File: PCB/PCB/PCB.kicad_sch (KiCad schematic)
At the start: 53 parts, among them J1 AudioJack Right, J2 USB_B_Micro, J3 AudioJack Left, J4 6PIN DISPLAY CONNECTOR, J5 CONN BAT, Q1 BC817, Q2 BC817, Q3 BSS84, U1 ESP32-S3-WROOM-1, U2 CP2102N-Axx-xQFN28, U3 NCP1117-3.3_SOT223, U4 UDA1334ATS, U5 PAM8403D, U6 MCP73831-3-OT

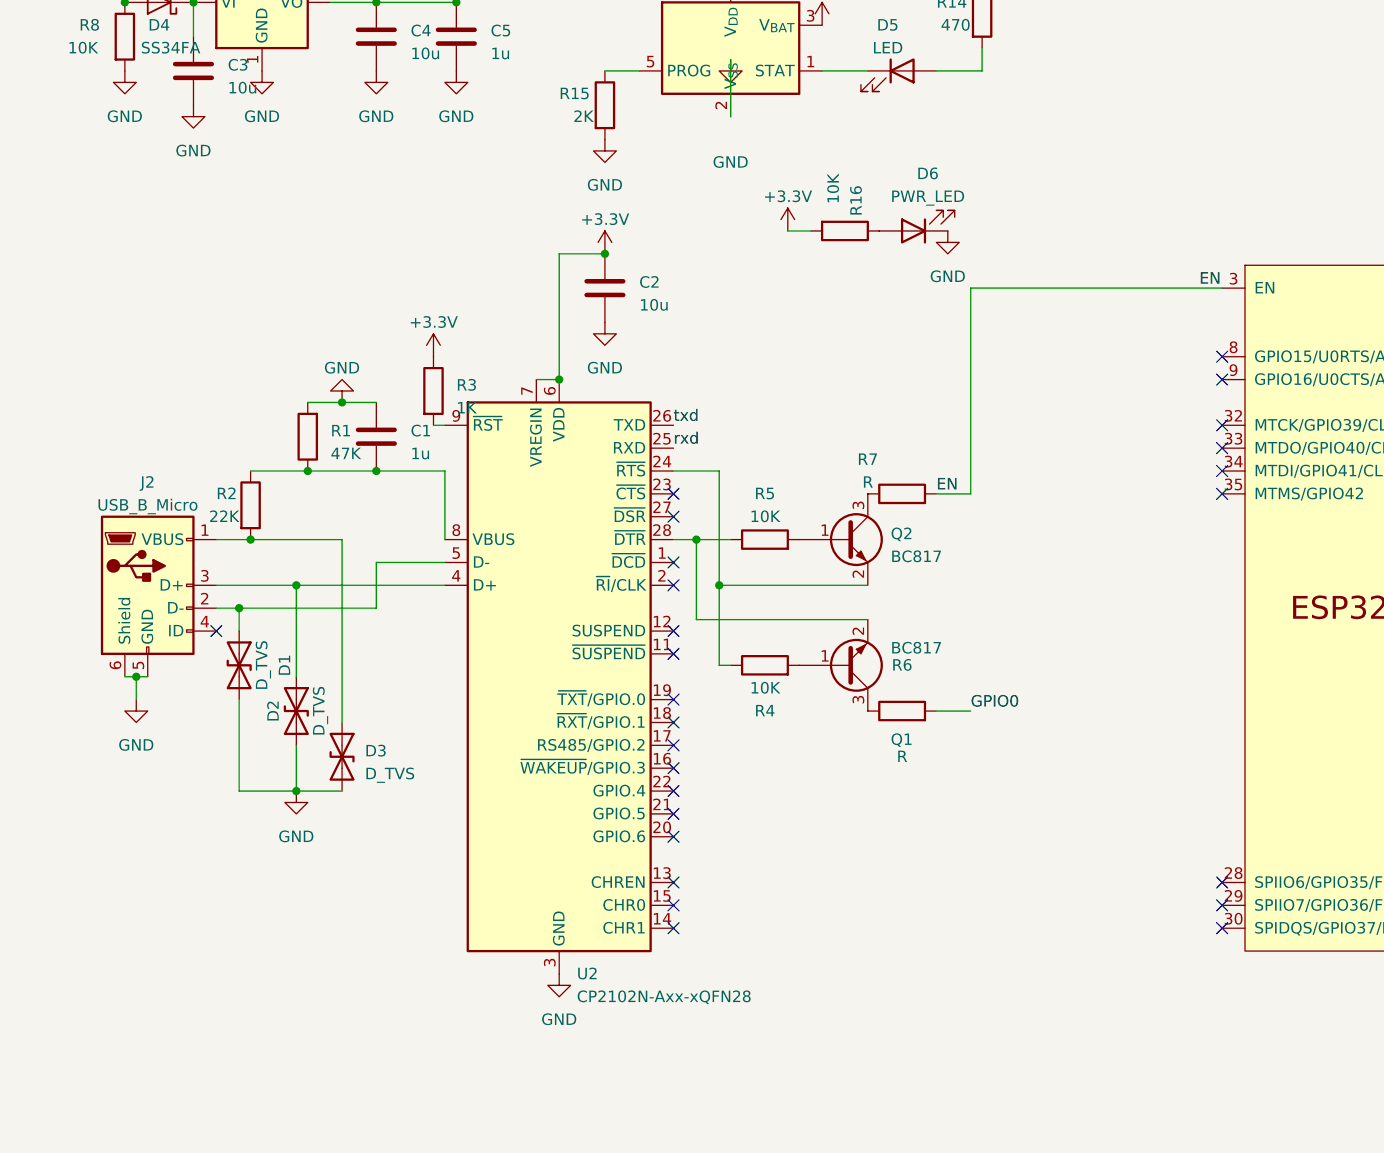
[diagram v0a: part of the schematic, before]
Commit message: PCB finished
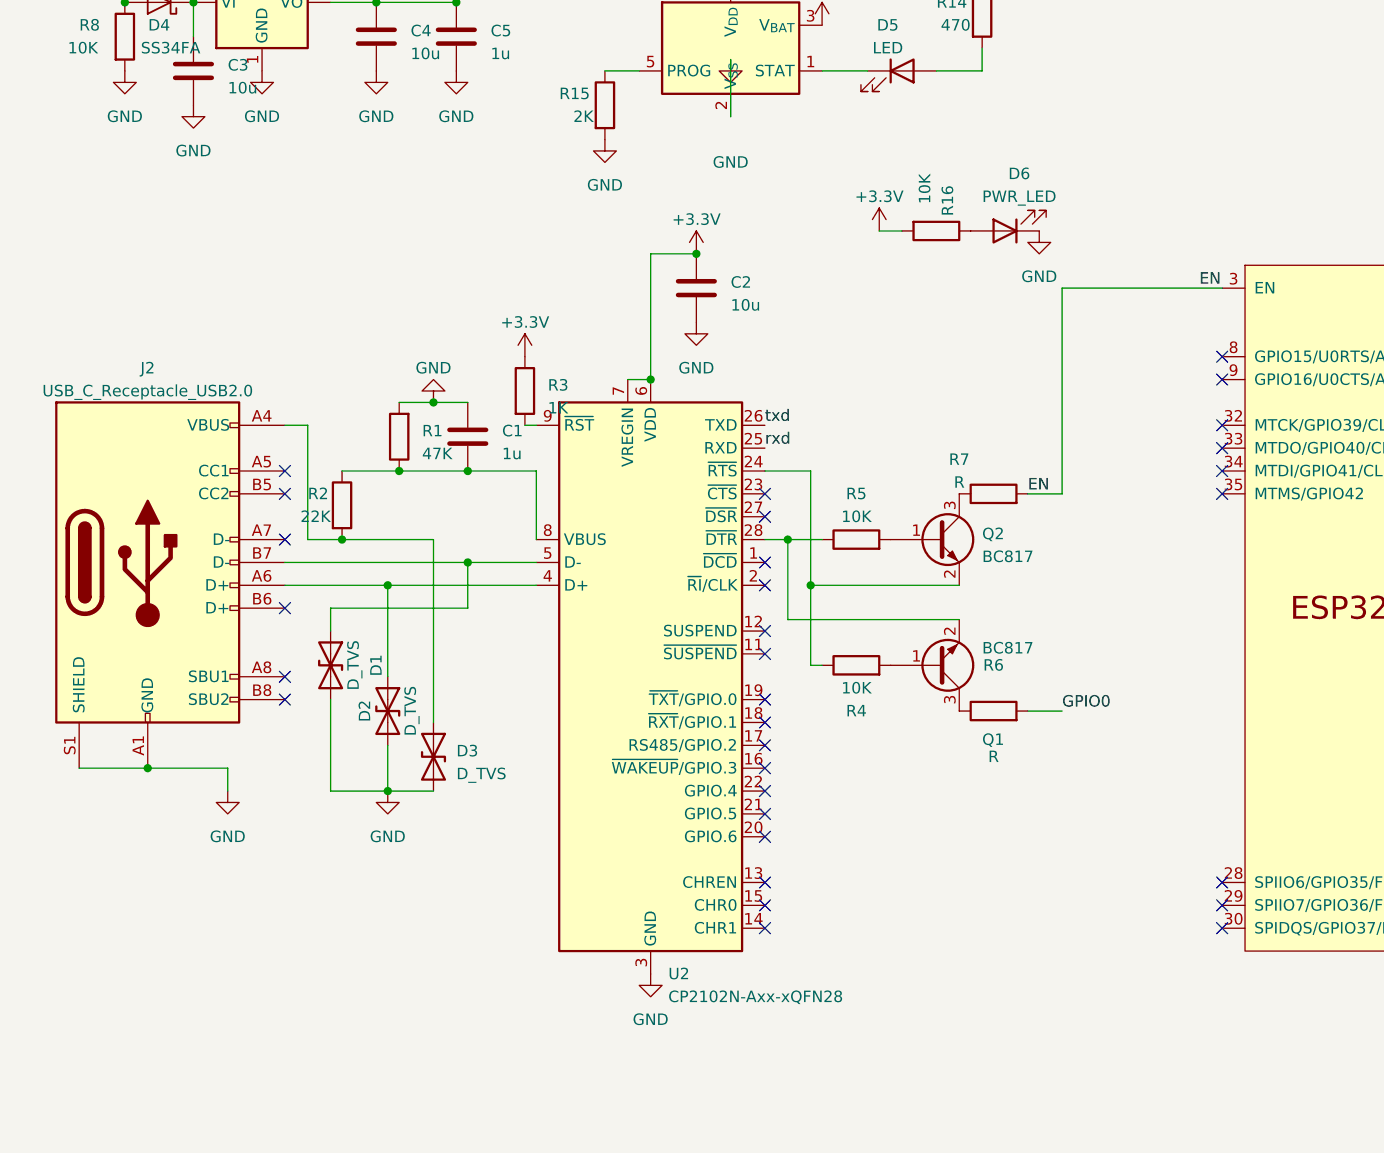
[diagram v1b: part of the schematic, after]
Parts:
- removed J2: USB_B_Micro, Connector_USB:USB_Micro-B_Molex-105017-0001, symbol Connector:USB_B_Micro
- added J2: USB_C_Receptacle_USB2.0, Connector_USB:USB_C_Receptacle_GCT_USB4105-xx-A_16P_TopMnt_Horizontal, symbol Connector:USB_C_Receptacle_USB2.0
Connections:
- net GND: now also J2.A1 (GND), J2.A12 (GND), J2.B1 (GND), J2.B12 (GND), J2.S1 (SHIELD)
- net at D3.1 (A1), R2.2: now also J2.A4 (VBUS), J2.A9 (VBUS), J2.B4 (VBUS), J2.B9 (VBUS)
- net at D1.1 (A1), U2.5 (D-): now also J2.B7 (D-)
- net at D2.1 (A1), U2.4 (D+): now also J2.A6 (D+)
- no-connect marks 44 -> 49
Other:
- moved on the sheet: C1, C2, D1, D2, D3, D6, Q1, Q2, R1, R16, R2, R3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
